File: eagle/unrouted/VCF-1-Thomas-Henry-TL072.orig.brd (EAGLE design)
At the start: 88.9 x 91.4 mm, 51 parts, among them IC1 TL072P, IC2 TL072P, IC3 LM13600, IC4 TL072P, J1 SPAD+--+, J2 SPAD+--+, J3 SPAD+--+, J4 SPAD+--+, J5 SPAD+--+, J6 SPAD+--+, T1 2N3906, T2 2N3906

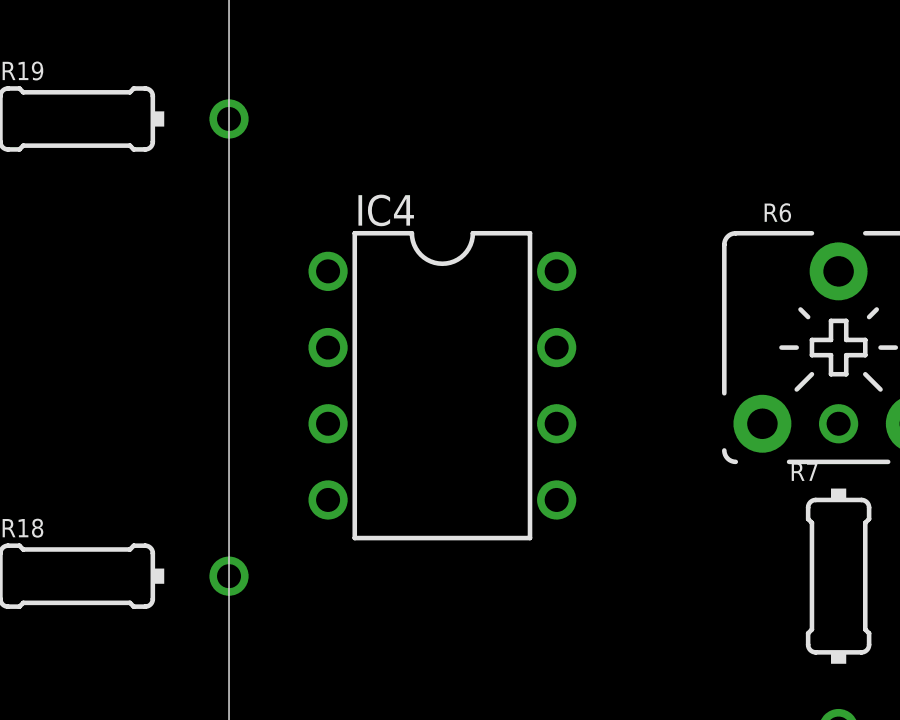
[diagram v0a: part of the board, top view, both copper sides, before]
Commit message: ...
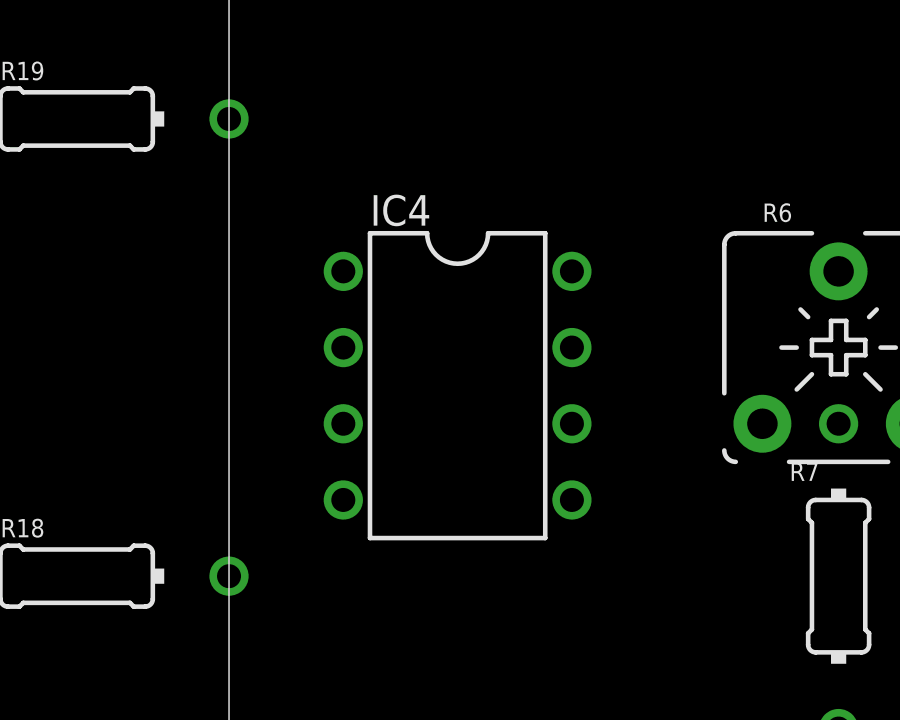
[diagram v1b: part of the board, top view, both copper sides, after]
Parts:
- moved IC4 0.51 mm to (7.62, 41.9)
